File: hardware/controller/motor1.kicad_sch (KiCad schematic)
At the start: 56 parts, among them J5 Conn_01x01, J6 Conn_01x01, J7 Conn_01x01, J8 Conn_01x06, J9 Conn_01x03, Q2 AOD66406, Q3 AOD66406, Q4 AOD66406, Q5 AOD66406, Q6 AOD66406, Q7 AOD66406, U10 MCP6541, U11 LM2105D, U12 MCP6541, U13 LM2105D, U8 MCP6541, U9 LM2105D

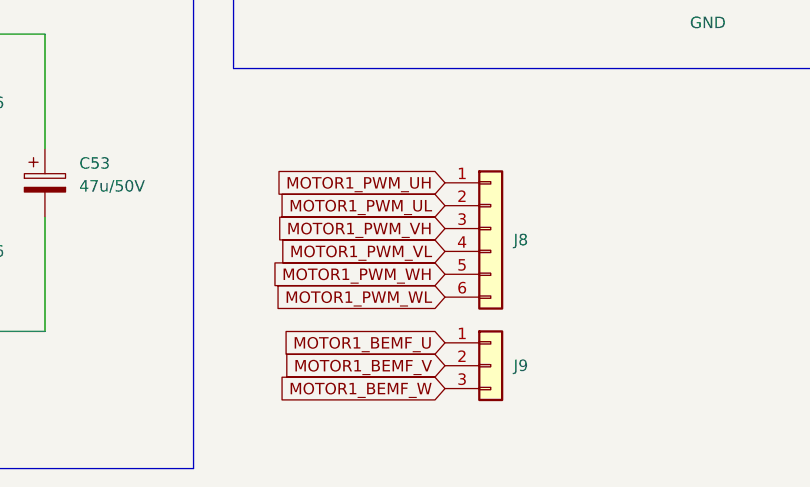
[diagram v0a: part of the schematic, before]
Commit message: wip - placement
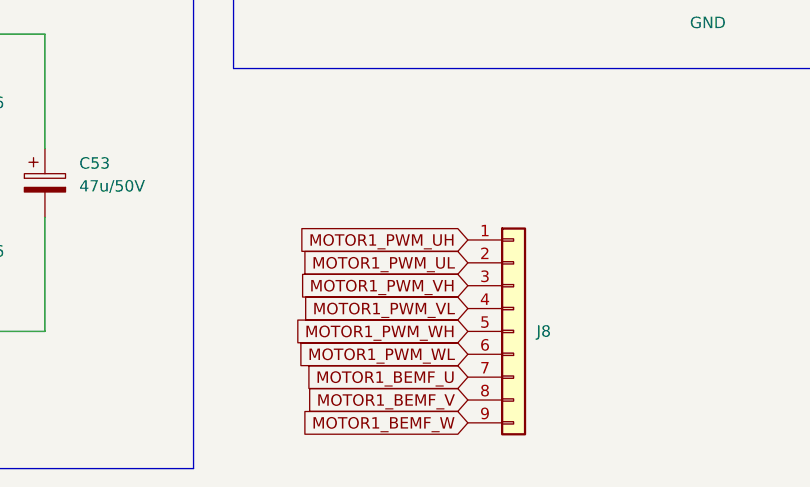
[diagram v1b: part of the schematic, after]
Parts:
- removed J8: Conn_01x06, Connector_PinHeader_2.54mm:PinHeader_1x06_P2.54mm_Vertical, symbol Connector_Generic:Conn_01x06
- removed J9: Conn_01x03, Connector_PinHeader_2.54mm:PinHeader_1x03_P2.54mm_Vertical, symbol Connector_Generic:Conn_01x03
- added J8: Conn_01x09, Connector_PinHeader_2.54mm:PinHeader_1x09_P2.54mm_Vertical, symbol Connector_Generic:Conn_01x09
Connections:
- net MOTOR1_BEMF_U: now also J8.7 (Pin_7)
- net MOTOR1_BEMF_V: now also J8.8 (Pin_8)
- net MOTOR1_BEMF_W: now also J8.9 (Pin_9)
- net MOTOR1_PWM_UH: now also J8.1 (Pin_1)
- net MOTOR1_PWM_UL: now also J8.2 (Pin_2)
- net MOTOR1_PWM_VH: now also J8.3 (Pin_3)
- net MOTOR1_PWM_VL: now also J8.4 (Pin_4)
- net MOTOR1_PWM_WH: now also J8.5 (Pin_5)
- net MOTOR1_PWM_WL: now also J8.6 (Pin_6)
